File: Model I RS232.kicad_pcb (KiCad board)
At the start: 2 copper layers, 114.2 x 74 mm, 29 parts, among them U1 HD6402, U10 74LS08, U2 COM8116, U3 74LS155, U4 74LS04, U5 74LS00, U6 74LS244, U7 74LS367, U8 74LS174, U9 SP3243ECA-L/TR, Y1 5.0688 MHz

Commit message: Add files via upload
Updated local footprint for J1
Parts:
- J1: footprint Byteshift_Library:TRS-80 M1 EI_ADDON_42P_CONN -> ModelIRS232:TRS-80 M1 EI_ADDON_42P_CONN

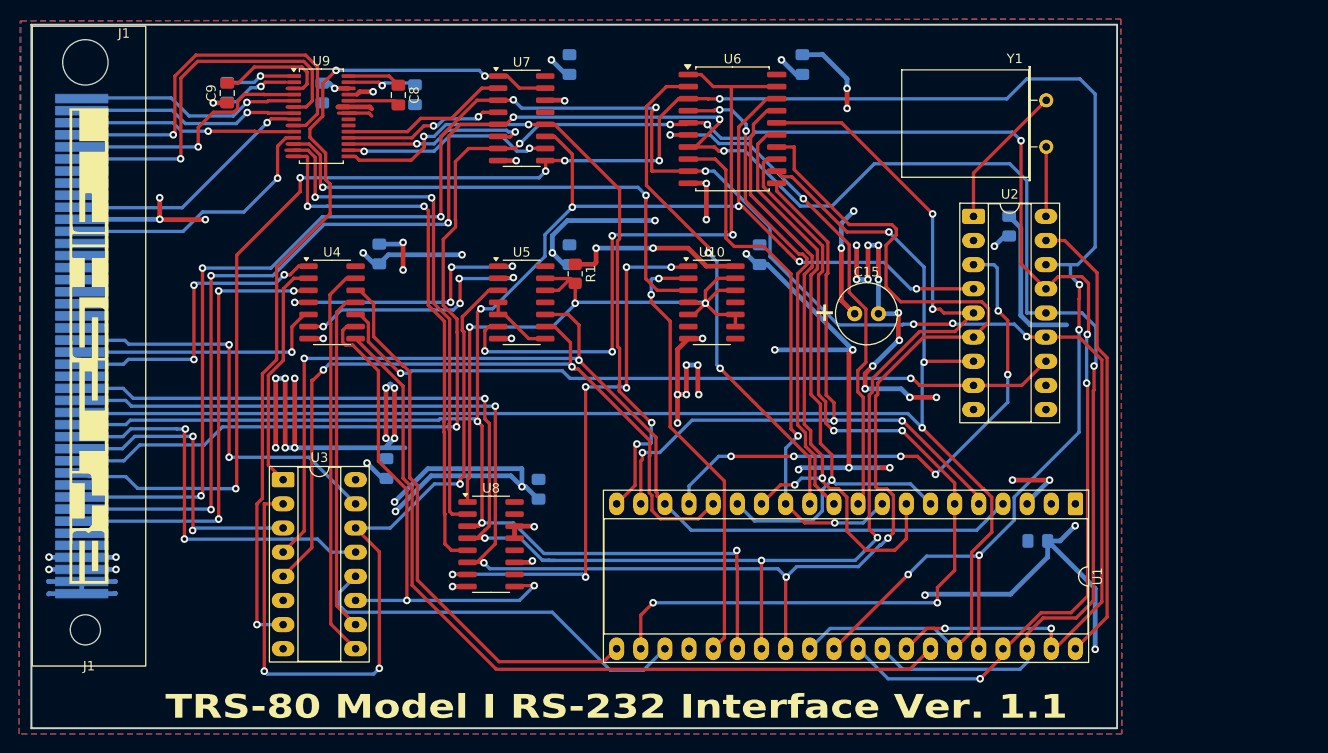
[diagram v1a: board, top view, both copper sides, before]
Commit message: Add files via upload
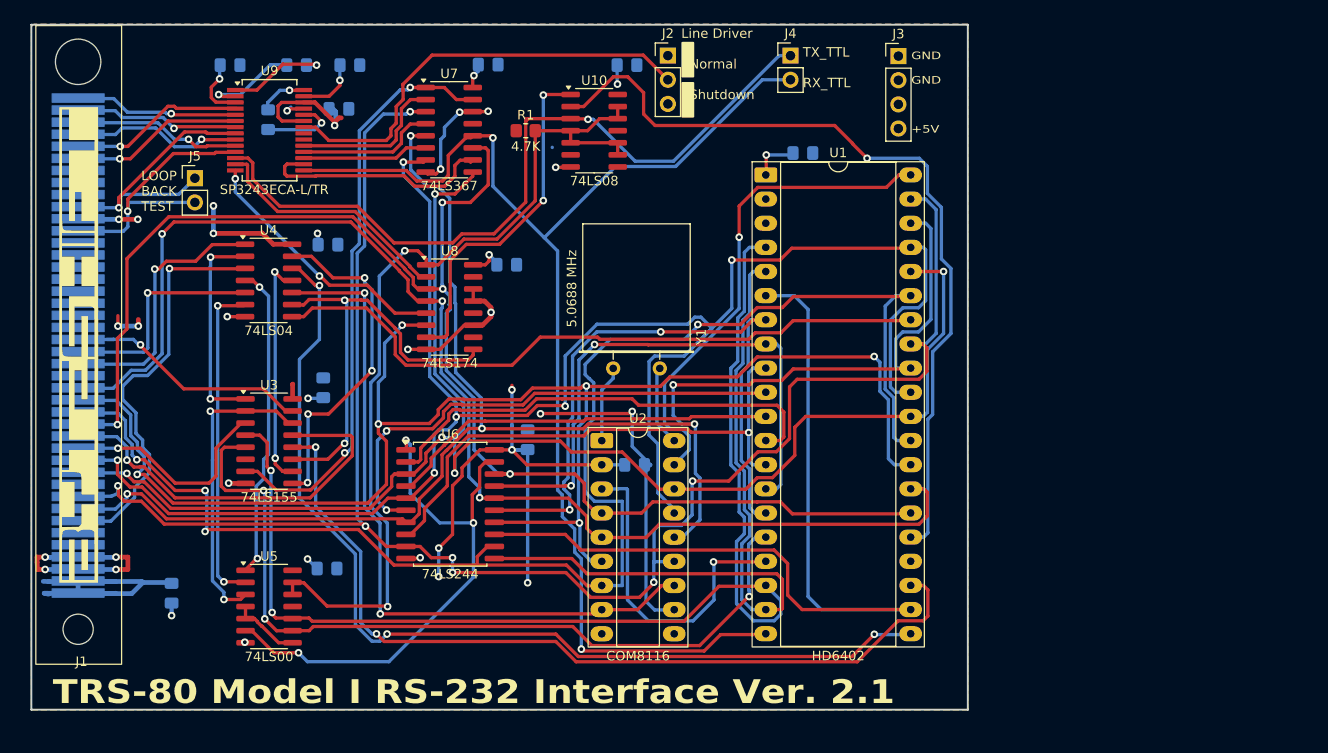
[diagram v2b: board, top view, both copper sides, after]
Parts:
- added J2: Conn_01x03_Pin, Connector_PinHeader_2.54mm:PinHeader_1x03_P2.54mm_Vertical, F.Cu at (142.8, 77.8)
- added J3: Conn_01x04_Pin, Connector_PinHeader_2.54mm:PinHeader_1x04_P2.54mm_Vertical, F.Cu at (167.1, 77.9)
- added J4: Conn_01x02_Pin, Connector_PinHeader_2.54mm:PinHeader_1x02_P2.54mm_Vertical, F.Cu at (155.8, 77.8)
- added J5: Conn_01x02_Pin, Connector_PinHeader_2.54mm:PinHeader_1x02_P2.54mm_Vertical, F.Cu at (93.1, 90.8)
- C11: value 0.47uF -> 0.1uF
- C15: footprint Capacitor_THT:C_Radial_D6.3mm_H11.0mm_P2.50mm -> Capacitor_SMD:C_0805_2012Metric_Pad1.18x1.45mm_HandSolder; moved to B.Cu
- C8, C9: moved to B.Cu
- J1: footprint ModelIRS232:TRS-80 M1 EI_ADDON_42P_CONN -> Byteshift_Library:TRS-80 M1 EI_ADDON_42P_CONN
- U3: footprint Package_DIP:DIP-16_W7.62mm_Socket_LongPads -> Package_SO:SOIC-16_3.9x9.9mm_P1.27mm
- U9: footprint Package_SO:TSSOP-28_4.4x9.7mm_P0.65mm -> Package_SO:SSOP-28_5.3x10.2mm_P0.65mm
- moved C15 77.6 mm to (90.7, 134.4), turned to 90 degrees
- moved Y1 49.5 mm to (142.0, 110.8), turned to 180 degrees
- moved U6 49.4 mm to (120.0, 125.0)
- moved C6 48.9 mm to (128.1, 118.2)
- moved C1 47.7 mm to (157.1, 88.1), turned to 0 degrees
- moved U1 47.5 mm to (153.2, 90.4), turned to 0 degrees
- moved C5 46.7 mm to (139.3, 120.9), turned to 0 degrees
- moved U2 45.7 mm to (135.9, 118.3)
- moved C12 41.7 mm to (107.0, 131.8), turned to 0 degrees
- moved U5 41.6 mm to (100.9, 135.8)
- moved U8 25.3 mm to (119.9, 104.3)
- moved C14 24.3 mm to (138.6, 78.8), turned to 0 degrees
- moved C7 23.8 mm to (125.9, 99.8), turned to 0 degrees
- moved U10 21.9 mm to (135.1, 85.8)
- moved R1 15.9 mm to (127.9, 85.8), turned to 0 degrees
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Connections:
- net Net-(U1-RX_SERIAL) renamed RX_TTL
- net Net-(U9-T3IN) renamed TX_TTL
- U9 pad 22: VCC -> ~{SHUTDOWN}
- Y1 pad 1: Net-(U2-XTAL/EXT1) -> Net-(U2-XTAL/EXT2)
- Y1 pad 2: Net-(U2-XTAL/EXT2) -> Net-(U2-XTAL/EXT1)
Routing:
- net GND: track 195.4 -> 107.9 mm, vias 49 -> 15
- net VCC: track 205.2 -> 125.2 mm, vias 29 -> 22
- net D4: track 230.5 -> 159.4 mm, vias 10 -> 5
- net RX_TTL: track 70.2 -> 134.9 mm, vias 4 -> 2
- net D6: track 227.8 -> 174.6 mm, vias 7 -> 5
- net Net-(U3-Ea2): track 83.5 -> 31.6 mm, vias 3 -> 2
- net Net-(U1-~{TXLOAD}): track 41.8 -> 91.0 mm, vias 0 -> 2
- net ~{SHUTDOWN}: track 0.00 -> 46.1 mm
- net D1: track 180.2 -> 134.4 mm, vias 6 -> 3
- net Net-(U1-RESET): track 58.5 -> 103.3 mm, vias 0 -> 3
- net Net-(U1-TX_SERIAL): track 46.5 -> 85.7 mm, vias 2 -> 1
- net D0: track 190.3 -> 152.9 mm, vias 8 -> 4
- net Net-(U8-Q1): track 58.7 -> 27.6 mm
- net Net-(U8-Q0): track 55.0 -> 24.6 mm, vias 2 -> 0
- net Net-(U3-Q0a): track 89.0 -> 62.0 mm, vias 3 -> 2
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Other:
- board size 114.2 x 74 mm -> 98.5 x 72.1 mm
- board text added: "GND GND +5V"
- board text added: "LOOP BACK TEST"
- board text added: "Line Driver Normal Shutdown"
- board text added: "TRS-80 Model I RS-232 Interface Ver. 2.1"
- board text added: "TX_TTL RX_TTL"
- board text added: "made in frustration"
- board text removed: "+"
- board text removed: "TRS-80 Model I RS-232 Interface Ver. 1.1"
